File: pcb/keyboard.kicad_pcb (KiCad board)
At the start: 2 copper layers, 106.9 x 64.7 mm, 23 parts

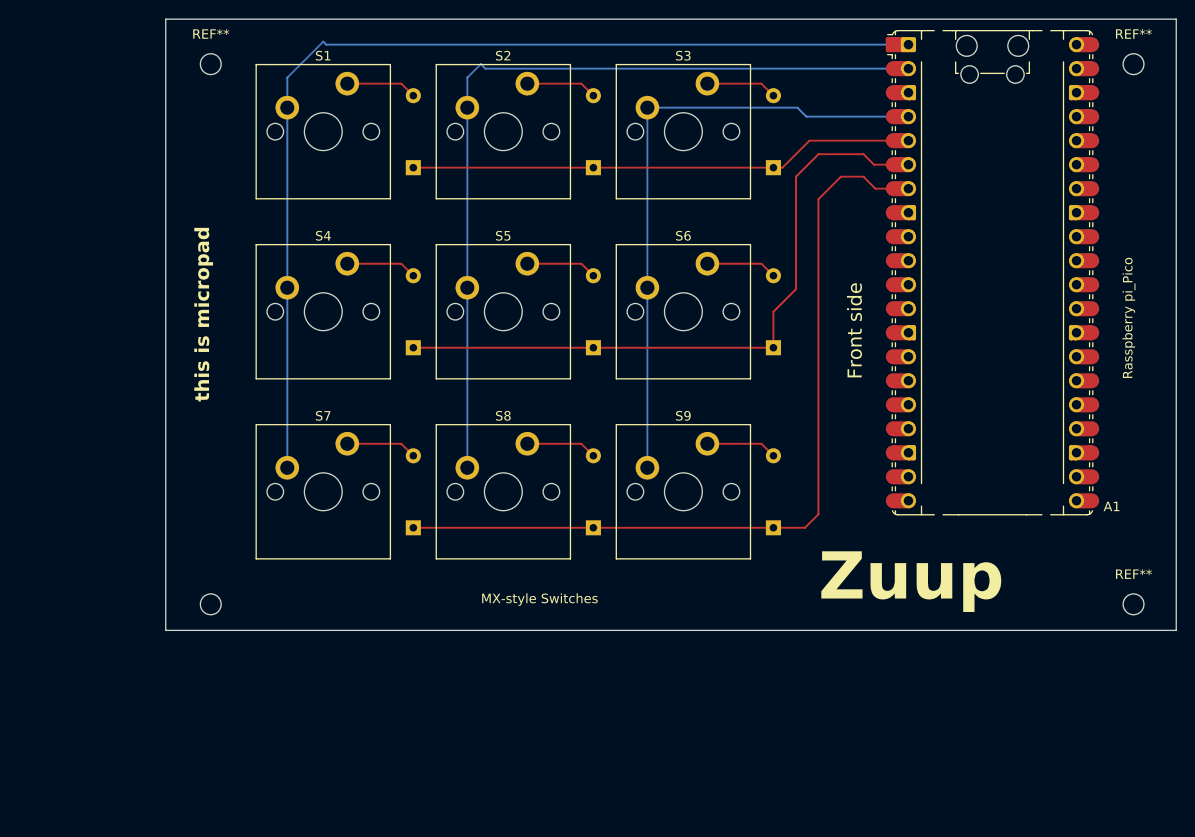
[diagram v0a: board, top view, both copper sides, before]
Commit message: oled screen a dial new case new pc
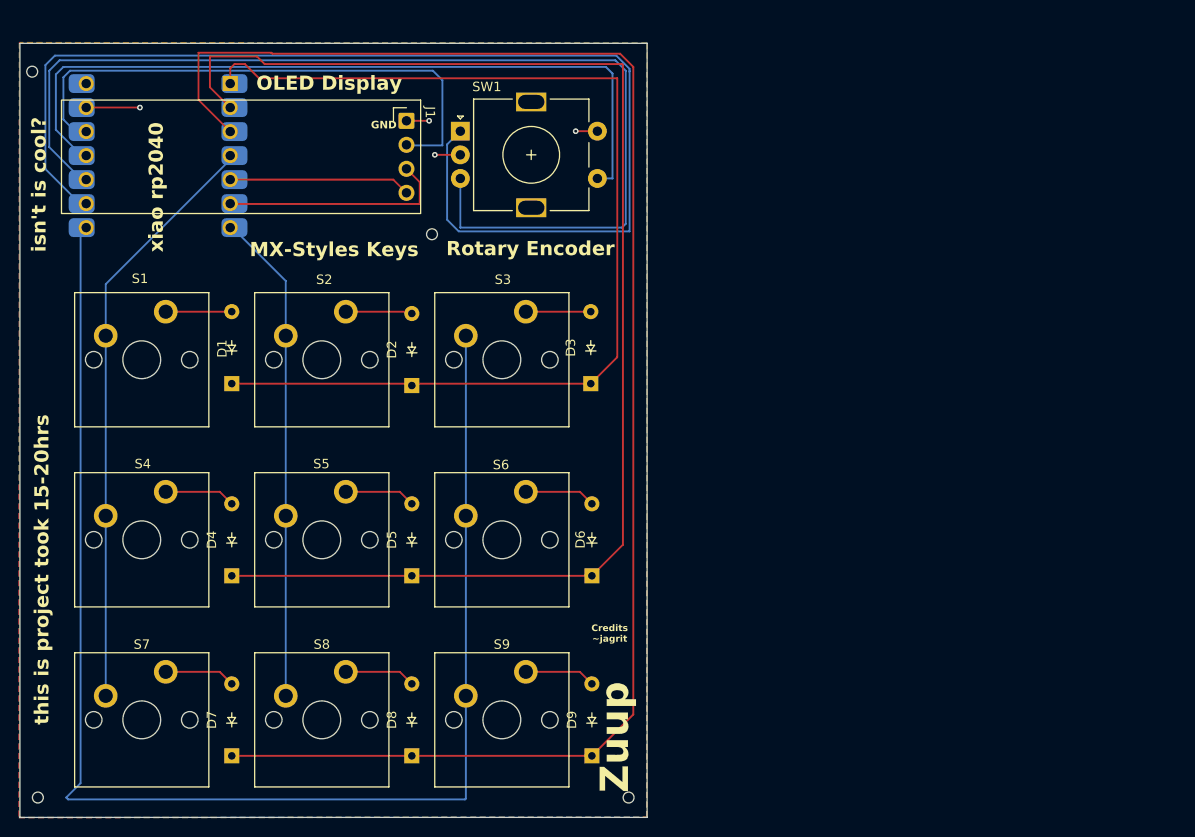
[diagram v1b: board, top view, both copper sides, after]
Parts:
- removed A1: RaspberryPi_Pico, Module:RaspberryPi_Pico_Common_Unspecified
- removed the REF** at (64.3, 50.0)
- removed the REF** at (161.9, 107.2)
- removed the REF** at (64.3, 107.2)
- removed the REF** at (161.9, 50.0)
- added J1: Conn_01x04_Pin, Display:ER_OLEDM0.91_1x-I2C, F.Cu at (85.0, 56.0)
- added REF**: ToolingHole_1.152mm, MountingHole:ToolingHole_1.152mm, F.Cu at (87.7, 68.0)
- added REF**: ToolingHole_1.152mm, MountingHole:ToolingHole_1.152mm, F.Cu at (46.0, 127.6)
- added REF**: ToolingHole_1.152mm, MountingHole:ToolingHole_1.152mm, F.Cu at (108.5, 127.6)
- added REF**: ToolingHole_1.152mm, MountingHole:ToolingHole_1.152mm, F.Cu at (45.4, 50.8)
- added SW1: RotaryEncoder_Switch, Rotary_Encoder:RotaryEncoder_Alps_EC11E-Switch_Vertical_H20mm, F.Cu at (90.7, 57.1)
- added U1: MCU_Seeed_XIAO_RP2040, ScottoKeebs_MCU:Seeed_XIAO_RP2040, B.Cu at (58.7, 59.7)
- D1, D2, D3, D4, D5, D6, D7, D8, D9: moved to F.Cu
- moved S1 30.8 mm to (57.0, 81.3)
- moved D5 30.8 mm to (85.6, 104.1)
- moved D6 30.8 mm to (104.6, 104.1)
- moved D8 30.8 mm to (85.6, 123.2)
- moved D9 30.8 mm to (104.6, 123.2)
- moved S2 30.8 mm to (76.0, 81.3)
- moved S3 30.8 mm to (95.1, 81.3)
- moved D4 30.8 mm to (66.5, 104.1)
- moved D7 30.8 mm to (66.5, 123.2)
- moved S4 30.8 mm to (57.0, 100.3)
- moved S5 30.8 mm to (76.0, 100.3)
- moved S6 30.8 mm to (95.1, 100.3)
- moved S7 30.8 mm to (57.0, 119.4)
- moved S8 30.8 mm to (76.0, 119.4)
- moved S9 30.8 mm to (95.1, 119.4)
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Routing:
- net ENC_A: track 0.00 -> 126.0 mm
- net ENC_B: track 0.00 -> 113.9 mm
- net col 2: track 66.1 -> 152.2 mm
- net Row 2: track 87.0 -> 169.2 mm
- net ENC_SW: track 0.00 -> 81.9 mm
- net Row 1: track 69.7 -> 143.9 mm
- net Row 0: track 52.8 -> 114.8 mm
- net 3V3: track 0.00 -> 57.7 mm
- net col 0: track 108.7 -> 62.7 mm
- net col 1: track 88.7 -> 51.7 mm
- net SCL: track 0.00 -> 24.3 mm
- net SDA: track 0.00 -> 19.2 mm
- net GND: track 0.00 -> 13.1 mm, vias 0 -> 4
- net Net-(D2-A): track 7.51 -> 6.80 mm
- net Net-(D3-A): track 7.51 -> 6.86 mm
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- added copper zone on B.Cu, net GND
- added copper zone on F.Cu, net GND
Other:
- board size 106.9 x 64.7 mm -> 66.4 x 81.9 mm
- board text added: "Credits ~jagrit"
- board text added: "GND"
- board text added: "MX-Styles Keys"
- board text added: "OLED Display"
- board text added: "Place here"
- board text added: "Rotary Encoder"
- board text added: "isn't is cool?"
- board text added: "this is project took 15-20hrs"
- board text added: "xiao rp2040"
- board text removed: "Front side"
- board text removed: "MX-style Switches"
- board text removed: "Rasspberry pi_Pico"
- board text removed: "this is micropad"
